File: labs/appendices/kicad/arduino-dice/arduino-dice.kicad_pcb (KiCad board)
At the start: 2 copper layers, 10 parts, among them IC1 ATMEGA328P-P, P1 CONN_01X02, SW1 SW_PUSH, Y1 16 MHz

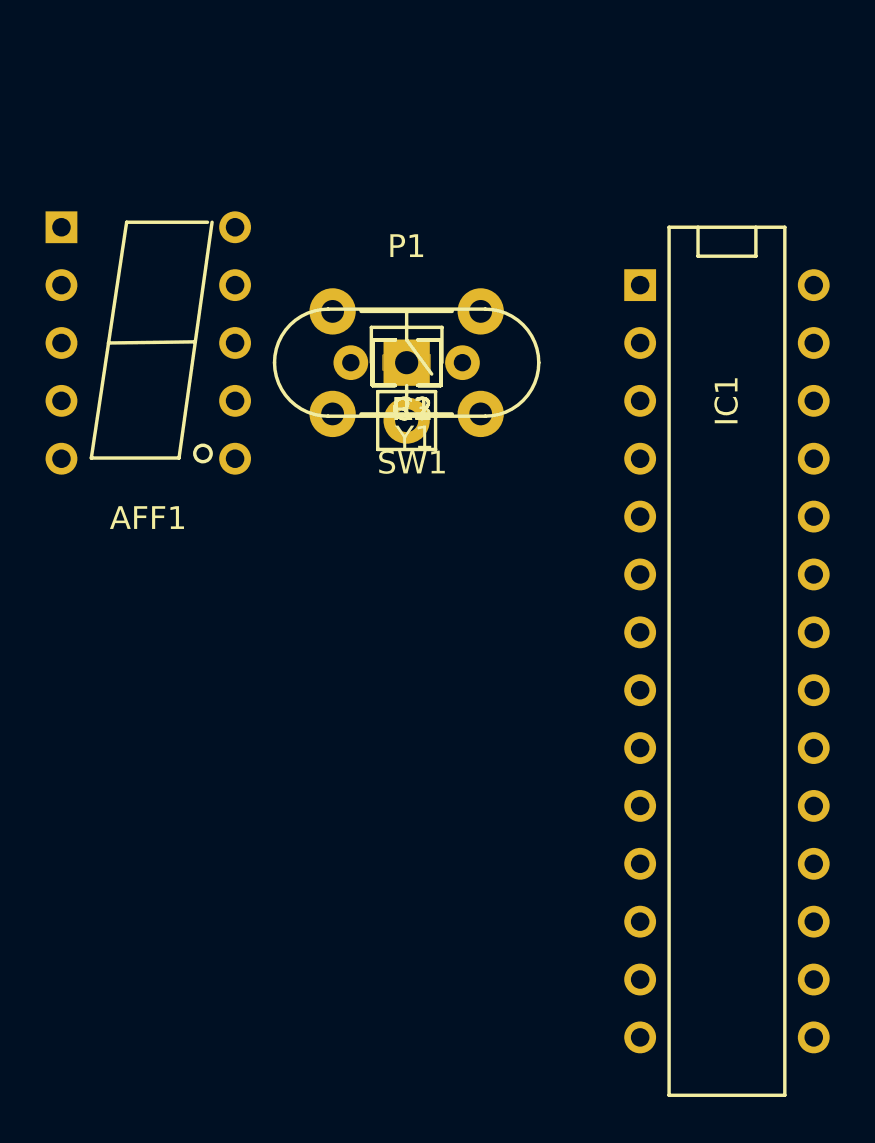
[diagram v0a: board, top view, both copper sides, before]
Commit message: update pcb
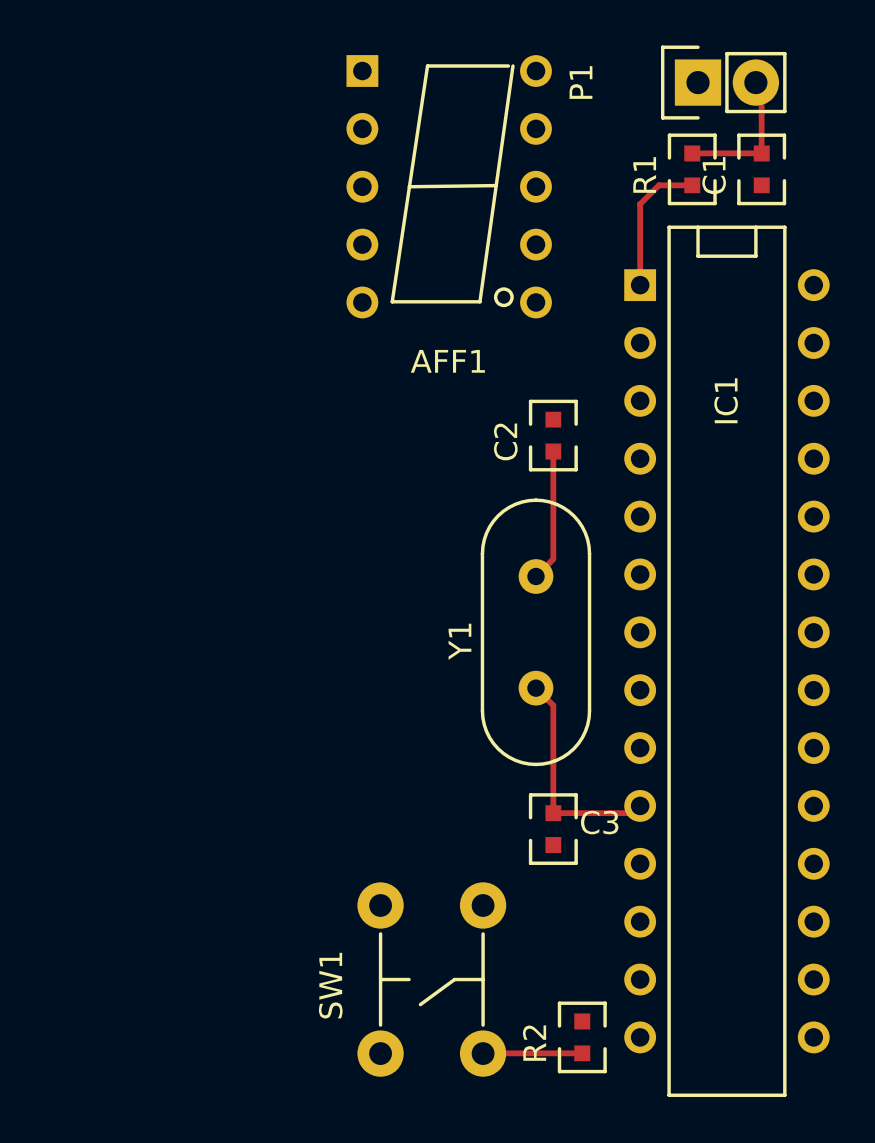
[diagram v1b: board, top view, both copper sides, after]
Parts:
- moved R2 30.6 mm to (156.2, 134.6), turned to 270 degrees
- moved SW1 27.1 mm to (149.6, 132.1), turned to 270 degrees
- moved C3 21.5 mm to (154.9, 125.5), turned to 90 degrees
- moved C1 17.7 mm to (164.1, 96.5), turned to 270 degrees
- moved P1 17.7 mm to (161.3, 92.7), turned to 90 degrees
- moved R1 15.1 mm to (161.0, 96.5), turned to 270 degrees
- moved AFF1 14.9 mm to (150.4, 97.3)
- moved Y1 13.1 mm to (154.2, 116.8), turned to 270 degrees
- moved C2 7.19 mm to (154.9, 108.2), turned to 270 degrees
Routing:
- net Net-(C3-Pad2): track 0.00 -> 9.74 mm
- net VCC: track 0.00 -> 6.26 mm
- net Net-(IC1-Pad1): track 0.00 -> 6.18 mm
- net Net-(C2-Pad2): track 0.00 -> 5.80 mm
- net /Button: track 0.00 -> 4.36 mm
